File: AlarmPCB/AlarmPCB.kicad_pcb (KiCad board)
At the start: 2 copper layers, 99.9 x 74 mm, 17 parts

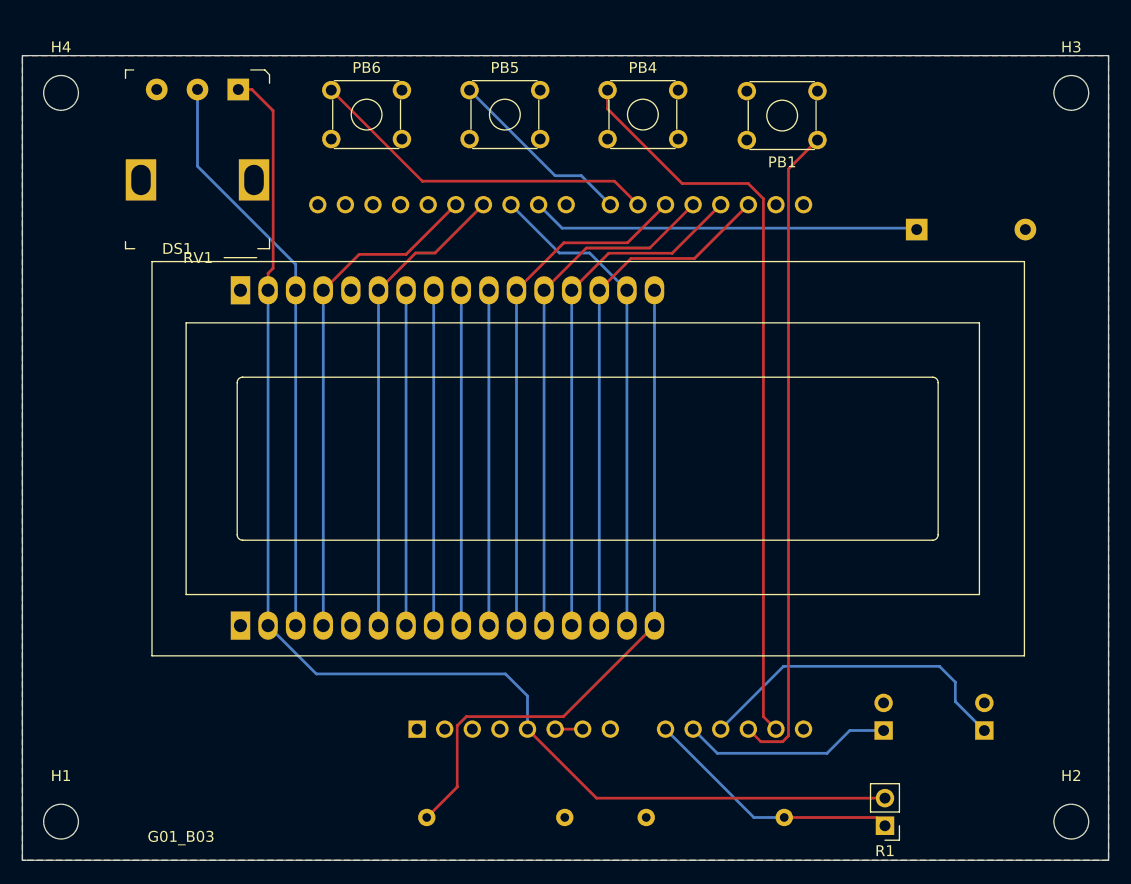
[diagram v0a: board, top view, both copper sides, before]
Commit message: Final PCB
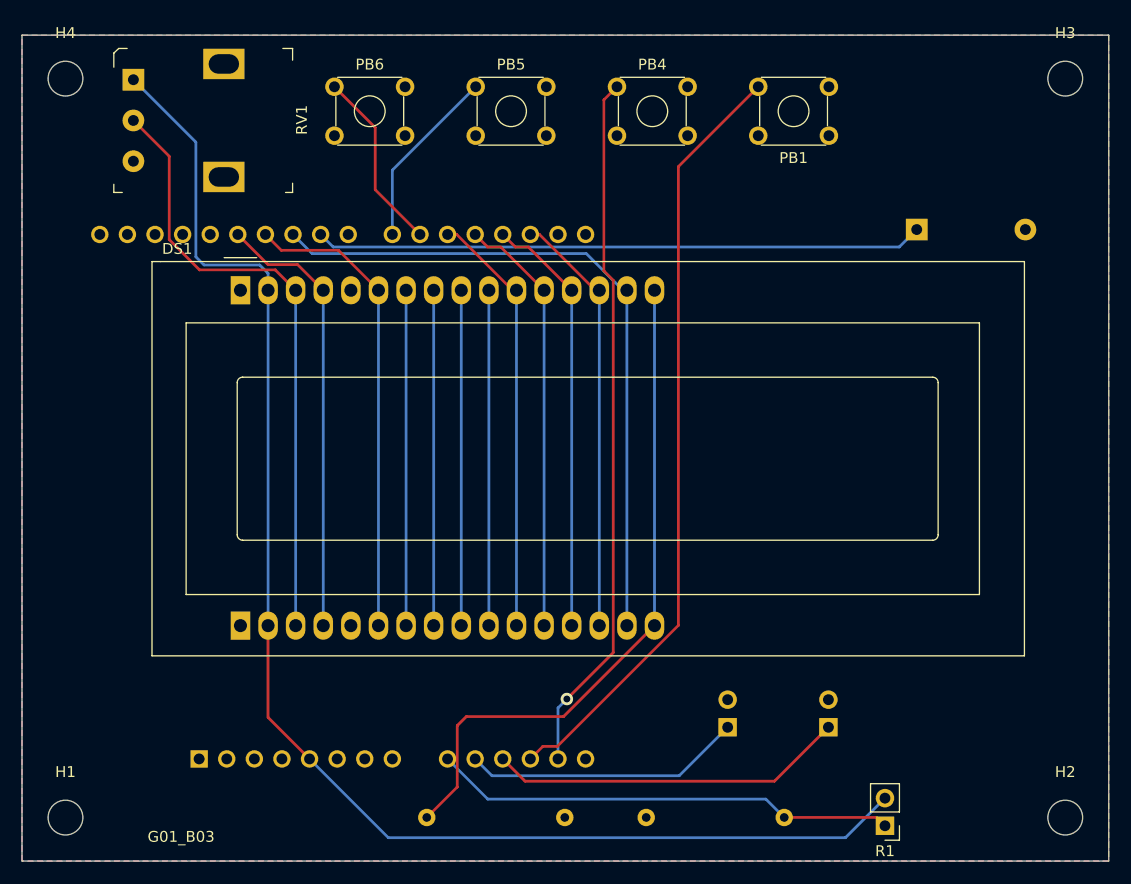
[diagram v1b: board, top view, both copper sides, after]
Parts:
- moved A1 20.2 mm to (88.4, 160.6)
- moved PB2 14.4 mm to (146.3, 157.7)
- moved PB3 14.4 mm to (137.0, 157.7)
- moved RV1 9.69 mm to (82.3, 98.1), turned to 270 degrees
- moved H3 1.43 mm to (168.1, 98.0)
- moved H4 1.38 mm to (76.1, 98.0)
- moved PB1 1.12 mm to (146.3, 103.2)
- moved PB4 0.92 mm to (126.8, 98.8)
- moved H2 0.67 mm to (168.1, 166.0)
- moved PB5 0.65 mm to (113.8, 98.8)
- moved H1 0.55 mm to (76.1, 166.0)
- moved PB6 0.42 mm to (100.8, 98.8)
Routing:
- net Net-(A1-Pad24): track 35.7 -> 56.0 mm
- net /D10: track 44.8 -> 63.7 mm
- net Net-(A1-Pad9): track 23.9 -> 42.8 mm
- net /D6: track 32.6 -> 16.8 mm
- net +5V: track 116.7 -> 129.7 mm
- net /A3: track 60.3 -> 71.3 mm
- net /D5: track 47.8 -> 39.3 mm
- net /D4: track 47.8 -> 39.3 mm
- net /D3: track 47.8 -> 39.3 mm
- net /D2: track 47.8 -> 39.3 mm
- net /A1: track 19.3 -> 25.7 mm
- net /D12: track 46.3 -> 40.8 mm
- net /A4: track 68.8 -> 64.8 mm, vias 0 -> 1
- net Net-(DS1-Pad3): track 53.1 -> 56.8 mm
- net /A2: track 30.1 -> 32.9 mm
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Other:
- board size 99.9 x 74 mm -> 100 x 76 mm
